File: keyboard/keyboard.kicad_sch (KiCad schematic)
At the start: 69 parts, among them U1 Pico

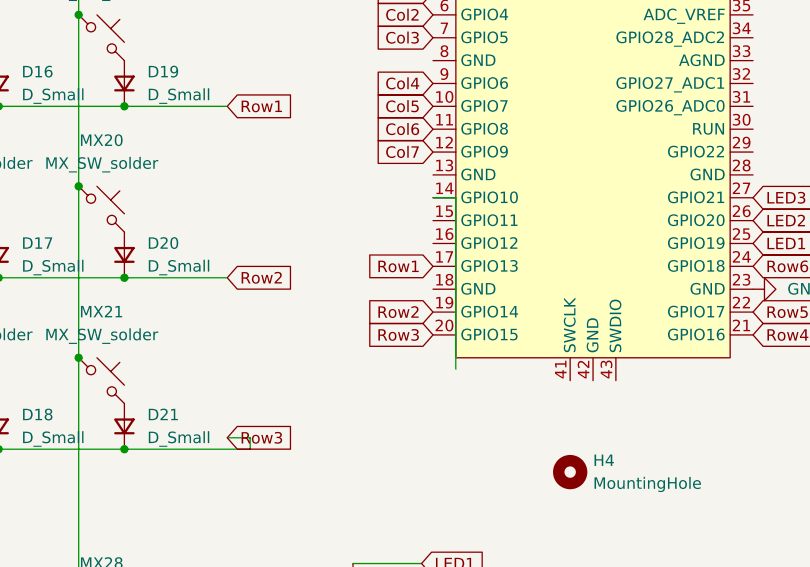
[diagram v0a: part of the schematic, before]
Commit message: writing
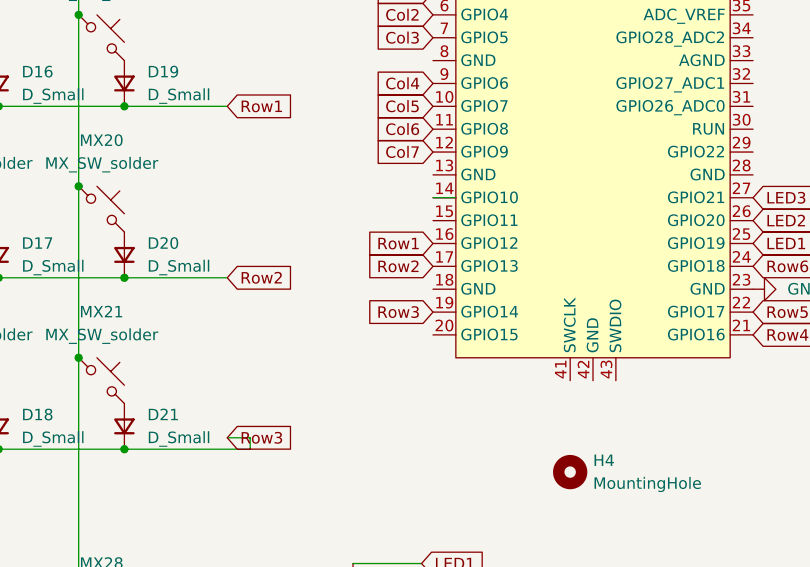
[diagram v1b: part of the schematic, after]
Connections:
- net Row1: now also U1.16 (GPIO12); no longer U1.17 (GPIO13)
- net Row2: now also U1.17 (GPIO13); no longer U1.19 (GPIO14)
- net Row3: now also U1.19 (GPIO14); no longer U1.20 (GPIO15)
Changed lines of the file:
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@@
-	(wire
-		(pts
-			(xy 189.23 82.55) (xy 189.23 63.5)
-		)
-		(stroke
-			(width 0)
-			(type default)
-		)
-	)
 	(wire
 		(pts
@@
 	(global_label "Row3"
 		(shape input)
-		(at 186.69 78.74 180)
+		(at 186.69 76.2 180)
 		(fields_autoplaced yes)
 		(effects
@@
 		)
 		(property "Intersheetrefs" "${INTERSHEET_REFS}"
-			(at 178.7458 78.74 0)
+			(at 178.7458 76.2 0)
 			(effects
 				(font
@@
 	(global_label "Row1"
 		(shape input)
+		(at 186.69 68.58 180)
+		(fields_autoplaced yes)
+		(effects
+			(font
+				(size 1.27 1.27)
+			)
+			(justify right)
+		)
+		(property "Intersheetrefs" "${INTERSHEET_REFS}"
+			(at 178.7458 68.58 0)
+			(effects
+				(font
+					(size 1.27 1.27)
+				)
+				(justify right)
+				(hide yes)
+			)
+		)
+	)
+	(global_label "Row5"
+		(shape input)
+		(at 165.1 138.43 0)
+		(fields_autoplaced yes)
+		(effects
+			(font
+				(size 1.27 1.27)
+			)
+			(justify left)
+		)
+		(property "Intersheetrefs" "${INTERSHEET_REFS}"
+			(at 173.0442 138.43 0)
+			(effects
+				(font
+					(size 1.27 1.27)
+				)
+				(justify left)
+				(hide yes)
+			)
+		)
+	)
+	(global_label "Row5"
+		(shape input)
+		(at 222.25 76.2 0)
+		(fields_autoplaced yes)
+		(effects
+			(font
+				(size 1.27 1.27)
+			)
+			(justify left)
+		)
+		(property "Intersheetrefs" "${INTERSHEET_REFS}"
+			(at 230.1942 76.2 0)
+			(effects
+				(font
+					(size 1.27 1.27)
+				)
+				(justify left)
+				(hide yes)
+			)
+		)
+	)
+	(global_label "LED3"
+		(shape input)
+		(at 185.42 142.24 0)
+		(fields_autoplaced yes)
+		(effects
+			(font
+				(size 1.27 1.27)
+			)
+			(justify left)
+		)
+		(property "Intersheetrefs" "${INTERSHEET_REFS}"
+			(at 193.0618 142.24 0)
+			(effects
+				(font
+					(size 1.27 1.27)
+				)
+				(justify left)
+				(hide yes)
+			)
+		)
+	)
+	(global_label "Col1"
+		(shape input)
+		(at 43.18 34.29 90)
+		(fields_autoplaced yes)
+		(effects
+			(font
+				(size 1.27 1.27)
+			)
+			(justify left)
+		)
+		(property "Intersheetrefs" "${INTERSHEET_REFS}"
+			(at 43.18 26.3458 90)
+			(effects
+				(font
+					(size 1.27 1.27)
+				)
+				(justify left)
+				(hide yes)
+			)
+		)
+	)
+	(global_label "Col4"
+		(shape input)
+		(at 186.69 50.8 180)
+		(fields_autoplaced yes)
+		(effects
+			(font
+				(size 1.27 1.27)
+			)
+			(justify right)
+		)
+		(property "Intersheetrefs" "${INTERSHEET_REFS}"
+			(at 179.4111 50.8 0)
+			(effects
+				(font
+					(size 1.27 1.27)
+				)
+				(justify right)
+				(hide yes)
+			)
+		)
+	)
+	(global_label "Row1"
+		(shape input)
+		(at 163.83 53.34 0)
+		(fields_autoplaced yes)
+		(effects
+			(font
+				(size 1.27 1.27)
+			)
+			(justify left)
+		)
+		(property "Intersheetrefs" "${INTERSHEET_REFS}"
+			(at 171.7742 53.34 0)
+			(effects
+				(font
+					(size 1.27 1.27)
+				)
+				(justify left)
+				(hide yes)
+			)
+		)
+	)
+	(global_label "Col5"
+		(shape input)
+		(at 119.38 35.56 90)
+		(fields_autoplaced yes)
+		(effects
+			(font
+				(size 1.27 1.27)
+			)
+			(justify left)
+		)
+		(property "Intersheetrefs" "${INTERSHEET_REFS}"
+			(at 119.38 28.2811 90)
+			(effects
+				(font
+					(size 1.27 1.27)
+				)
+				(justify left)
+				(hide yes)
+			)
+		)
+	)
+	(global_label "LED1"
+		(shape input)
+		(at 222.25 68.58 0)
+		(fields_autoplaced yes)
+		(effects
+			(font
+				(size 1.27 1.27)
+			)
+			(justify left)
+		)
+		(property "Intersheetrefs" "${INTERSHEET_REFS}"
+			(at 229.8918 68.58 0)
+			(effects
+				(font
+					(size 1.27 1.27)
+				)
+				(justify left)
+				(hide yes)
+			)
+		)
+	)
+	(global_label "Col5"
+		(shape input)
+		(at 186.69 53.34 180)
+		(fields_autoplaced yes)
+		(effects
+			(font
+				(size 1.27 1.27)
+			)
+			(justify right)
+		)
+		(property "Intersheetrefs" "${INTERSHEET_REFS}"
+			(at 179.4111 53.34 0)
+			(effects
+				(font
+					(size 1.27 1.27)
+				)
+				(justify right)
+				(hide yes)
+			)
+		)
+	)
+	(global_label "Row2"
+		(shape input)
 		(at 186.69 71.12 180)
 		(fields_autoplaced yes)
@@
 			(effects
 				(font
-					(size 1.27 1.27)
-				)
-				(justify right)
-				(hide yes)
-			)
-		)
-	)
-	(global_label "Row5"
-		(shape input)
-		(at 165.1 138.43 0)
-		(fields_autoplaced yes)
-		(effects
-			(font
-				(size 1.27 1.27)
-			)
-			(justify left)
-		)
-		(property "Intersheetrefs" "${INTERSHEET_REFS}"
-			(at 173.0442 138.43 0)
-			(effects
-				(font
-					(size 1.27 1.27)
-				)
-				(justify left)
-				(hide yes)
-			)
-		)
-	)
-	(global_label "Row5"
-		(shape input)
-		(at 222.25 76.2 0)
-		(fields_autoplaced yes)
-		(effects
-			(font
-				(size 1.27 1.27)
-			)
-			(justify left)
-		)
-		(property "Intersheetrefs" "${INTERSHEET_REFS}"
-			(at 230.1942 76.2 0)
-			(effects
-				(font
-					(size 1.27 1.27)
-				)
-				(justify left)
-				(hide yes)
-			)
-		)
-	)
-	(global_label "LED3"
-		(shape input)
-		(at 185.42 142.24 0)
-		(fields_autoplaced yes)
-		(effects
-			(font
-				(size 1.27 1.27)
-			)
-			(justify left)
-		)
-		(property "Intersheetrefs" "${INTERSHEET_REFS}"
-			(at 193.0618 142.24 0)
-			(effects
-				(font
-					(size 1.27 1.27)
-				)
-				(justify left)
-				(hide yes)
-			)
-		)
-	)
-	(global_label "Col1"
-		(shape input)
-		(at 43.18 34.29 90)
-		(fields_autoplaced yes)
-		(effects
-			(font
-				(size 1.27 1.27)
-			)
-			(justify left)
-		)
-		(property "Intersheetrefs" "${INTERSHEET_REFS}"
-			(at 43.18 26.3458 90)
-			(effects
-				(font
-					(size 1.27 1.27)
-				)
-				(justify left)
-				(hide yes)
-			)
-		)
-	)
-	(global_label "Col4"
-		(shape input)
-		(at 186.69 50.8 180)
-		(fields_autoplaced yes)
-		(effects
-			(font
-				(size 1.27 1.27)
-			)
-			(justify right)
-		)
-		(property "Intersheetrefs" "${INTERSHEET_REFS}"
-			(at 179.4111 50.8 0)
-			(effects
-				(font
-					(size 1.27 1.27)
-				)
-				(justify right)
-				(hide yes)
-			)
-		)
-	)
-	(global_label "Row1"
-		(shape input)
-		(at 163.83 53.34 0)
-		(fields_autoplaced yes)
-		(effects
-			(font
-				(size 1.27 1.27)
-			)
-			(justify left)
-		)
-		(property "Intersheetrefs" "${INTERSHEET_REFS}"
-			(at 171.7742 53.34 0)
-			(effects
-				(font
-					(size 1.27 1.27)
-				)
-				(justify left)
-				(hide yes)
-			)
-		)
-	)
-	(global_label "Col5"
-		(shape input)
-		(at 119.38 35.56 90)
-		(fields_autoplaced yes)
-		(effects
-			(font
-				(size 1.27 1.27)
-			)
-			(justify left)
-		)
-		(property "Intersheetrefs" "${INTERSHEET_REFS}"
-			(at 119.38 28.2811 90)
-			(effects
-				(font
-					(size 1.27 1.27)
-				)
-				(justify left)
-				(hide yes)
-			)
-		)
-	)
-	(global_label "LED1"
-		(shape input)
-		(at 222.25 68.58 0)
-		(fields_autoplaced yes)
-		(effects
-			(font
-				(size 1.27 1.27)
-			)
-			(justify left)
-		)
-		(property "Intersheetrefs" "${INTERSHEET_REFS}"
-			(at 229.8918 68.58 0)
-			(effects
-				(font
-					(size 1.27 1.27)
-				)
-				(justify left)
-				(hide yes)
-			)
-		)
-	)
-	(global_label "Col5"
-		(shape input)
-		(at 186.69 53.34 180)
-		(fields_autoplaced yes)
-		(effects
-			(font
-				(size 1.27 1.27)
-			)
-			(justify right)
-		)
-		(property "Intersheetrefs" "${INTERSHEET_REFS}"
-			(at 179.4111 53.34 0)
-			(effects
-				(font
-					(size 1.27 1.27)
-				)
-				(justify right)
-				(hide yes)
-			)
-		)
-	)
-	(global_label "Row2"
-		(shape input)
-		(at 186.69 76.2 180)
-		(fields_autoplaced yes)
-		(effects
-			(font
-				(size 1.27 1.27)
-			)
-			(justify right)
-		)
-		(property "Intersheetrefs" "${INTERSHEET_REFS}"
-			(at 178.7458 76.2 0)
-			(effects
-				(font
